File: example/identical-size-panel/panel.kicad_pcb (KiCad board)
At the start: 2 copper layers, 229 x 129 mm, 160 parts, among them J1 Conn_01x40_Female

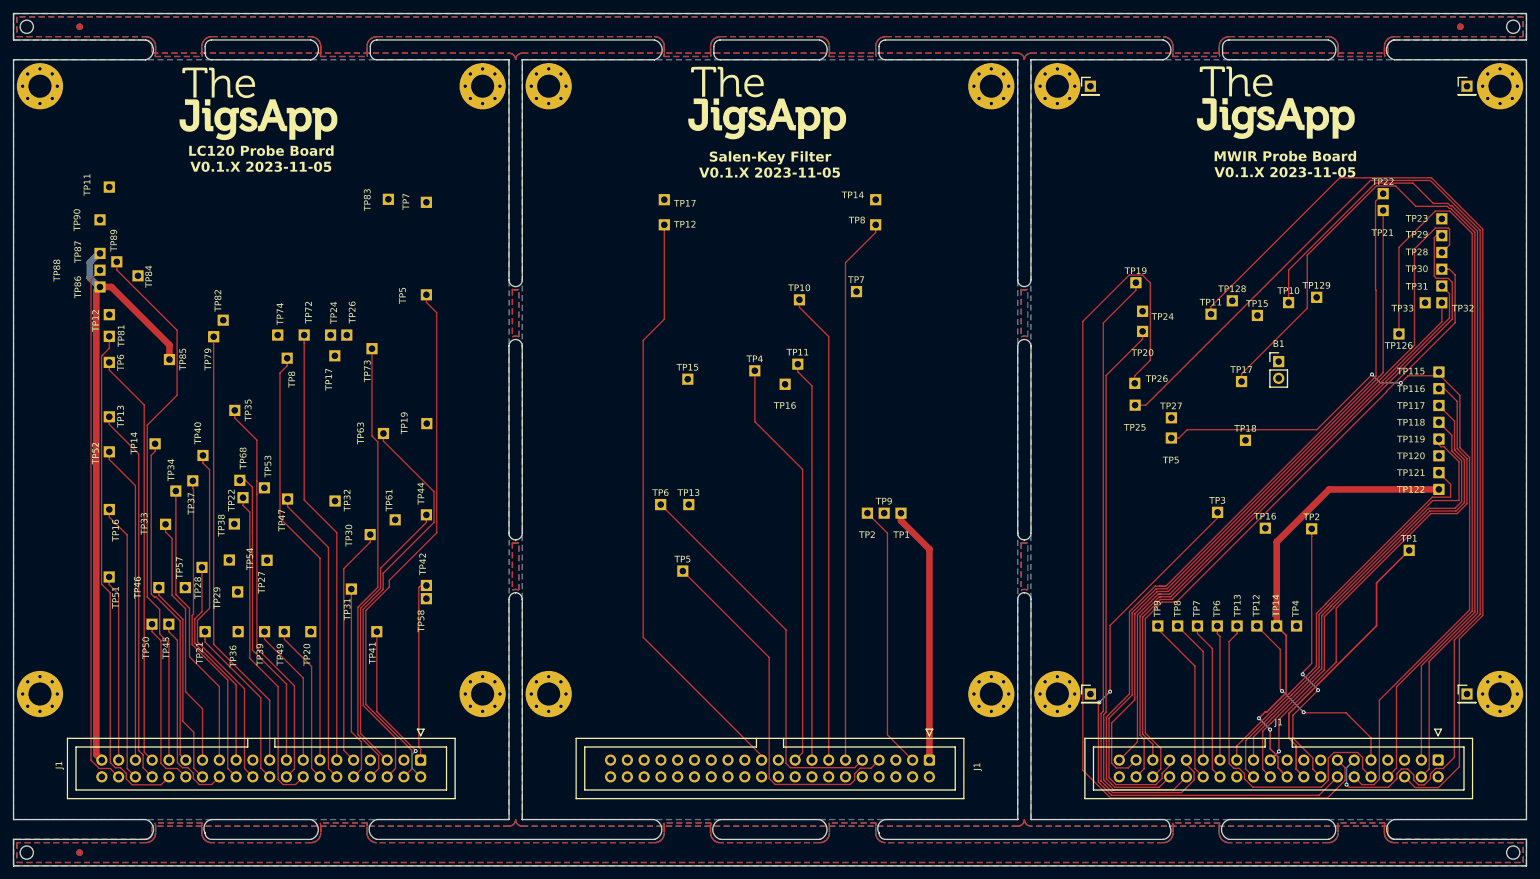
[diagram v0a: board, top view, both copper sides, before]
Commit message: updates
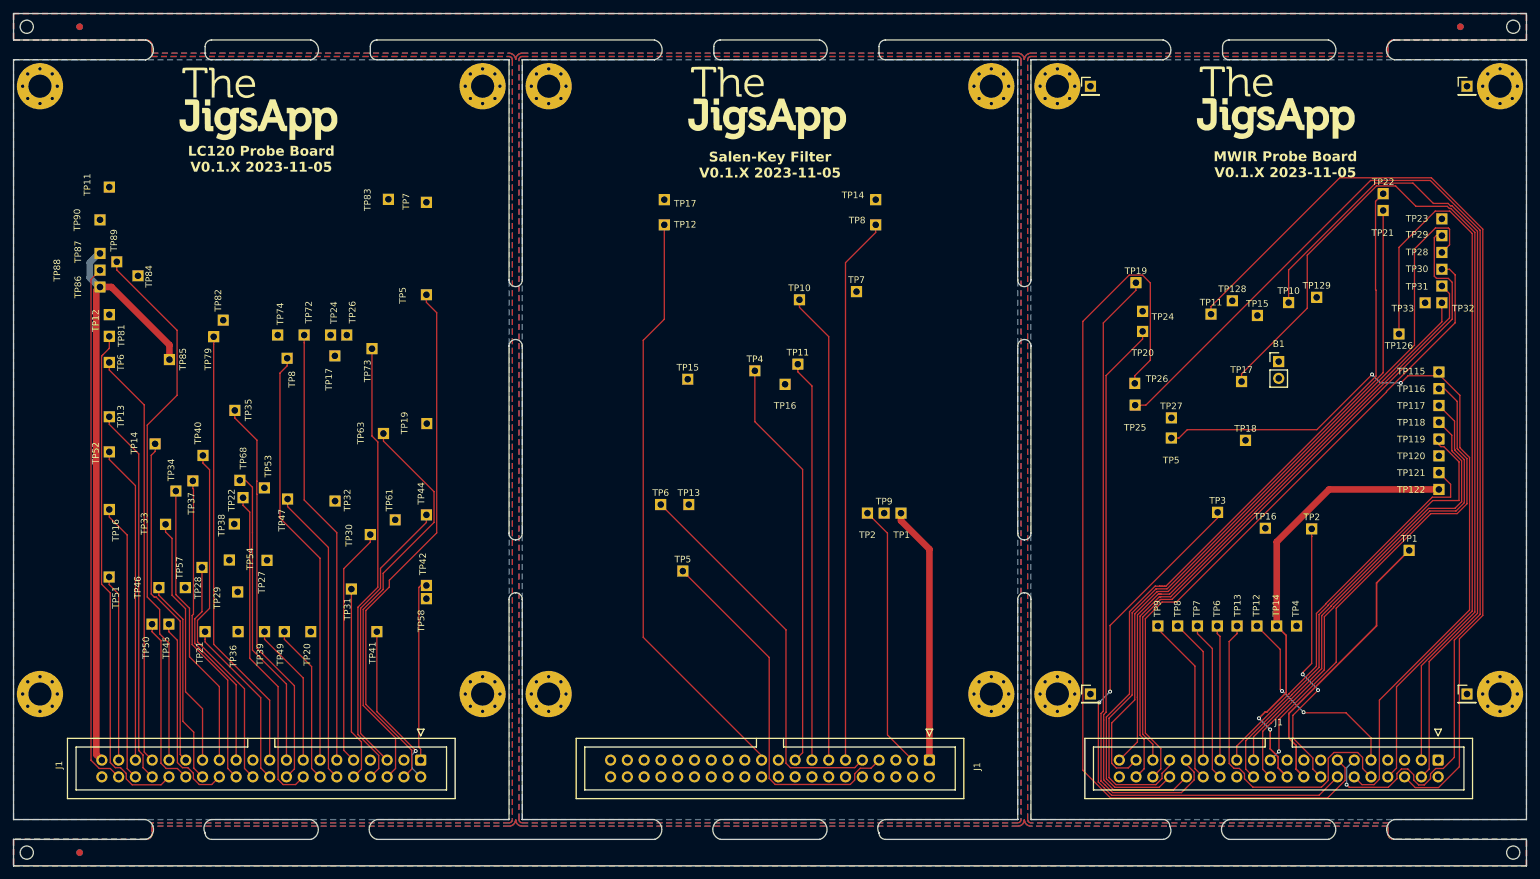
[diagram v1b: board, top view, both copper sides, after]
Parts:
- removed the G*** at (191.5, 5.83) (x2)
- removed the G*** at (37.5, 6.00) (x2)
- removed the G*** at (114.5, 5.88) (x2)
- removed KiKit_FID_B_1, KiKit_FID_B_2, KiKit_FID_B_3, KiKit_FID_T_1, KiKit_FID_T_2, KiKit_FID_T_3: Fiducial, Fiducial
- removed KiKit_TO_1, KiKit_TO_2, KiKit_TO_3, KiKit_TO_4: NPTH, NPTH
- added G***: LOGO, LOGO, F.Cu at (191.5, 5.83)
- added G***: LOGO, LOGO, F.Cu at (37.5, 6.00)
- added G***: LOGO, LOGO, F.Cu at (114.5, 5.88)
- added G***: LOGO, LOGO, B.Cu at (191.5, 5.83)
- added G***: LOGO, LOGO, B.Cu at (114.5, 5.88)
- added G***: LOGO, LOGO, B.Cu at (37.5, 6.00)
- added REF**: NPTH, NPTH, F.Cu at (2.00, -5.00)
- added REF**: Fiducial, Fiducial, B.Cu at (10.0, -5.00)
- added REF**: NPTH, NPTH, F.Cu at (2.00, 120.0)
- added REF**: Fiducial, Fiducial, F.Cu at (219.0, -5.00)
- added REF**: Fiducial, Fiducial, F.Cu at (10.0, -5.00)
- added REF**: NPTH, NPTH, F.Cu at (227.0, -5.00)
- added REF**: Fiducial, Fiducial, F.Cu at (10.0, 120.0)
- added REF**: NPTH, NPTH, F.Cu at (227.0, 120.0)
- added REF**: Fiducial, Fiducial, B.Cu at (10.0, 120.0)
- added REF**: Fiducial, Fiducial, B.Cu at (219.0, -5.00)
